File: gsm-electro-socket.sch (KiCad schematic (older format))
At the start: 18 parts, among them IC1 ATMEGA328-P, Q1 BC337, SW1 RESET, U1 PWRCONV, U2 SIM800C, Y1 16Mhz

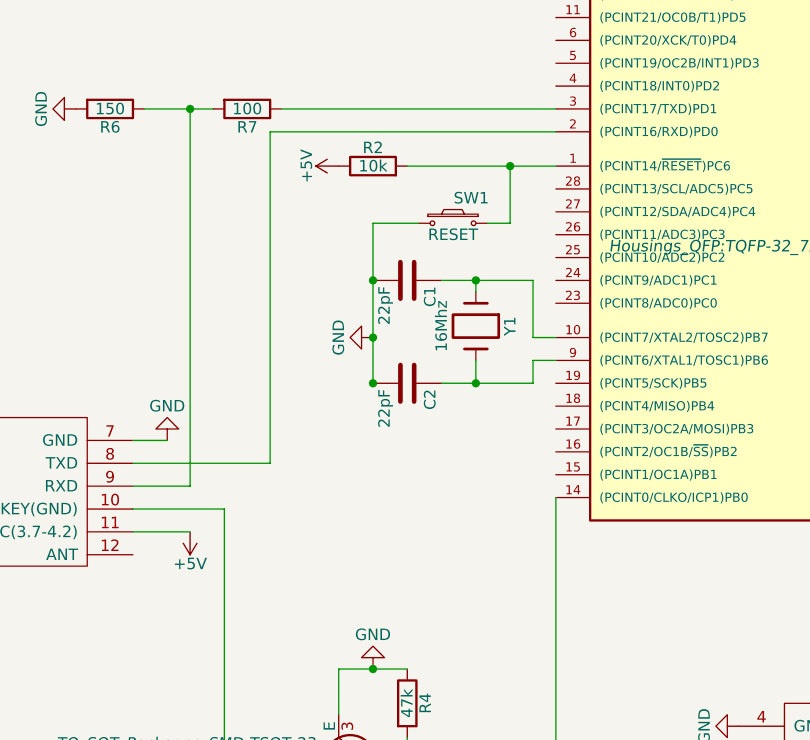
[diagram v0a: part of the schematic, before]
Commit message: update schema
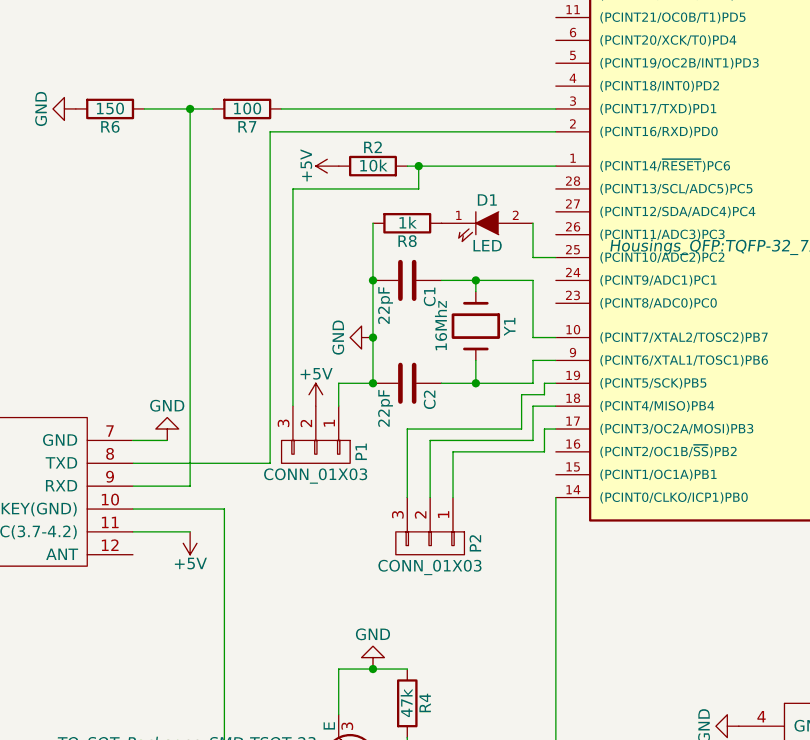
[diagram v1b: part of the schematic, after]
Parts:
- removed SW1: RESET, Buttons_Switches_SMD:SW_DIP_x1_W5.08mm_Slide_Copal_CHS-A, symbol SW_PUSH_SMALL_H
- added D1: LED, LEDs:LED_D2.0mm_W4.0mm_H2.8mm_FlatTop, symbol LED
- added P1, P2: CONN_01X03, Pin_Headers:Pin_Header_Angled_1x03_Pitch2.54mm, symbol CONN_01X03
- added R8: 1k, Resistors_SMD:R_0805_HandSoldering, symbol R
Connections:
- net +5V: now also P1.2 (P2)
- net GND: now also P1.1 (P1), R8.2
- net at IC1.1 ((PCINT14/~RESET~)PC6), R2.2: now also P1.3 (P3)
- net at IC1.17 ((PCINT3/OC2A/MOSI)PB3): now also P2.1 (P1)
- net at IC1.18 ((PCINT4/MISO)PB4): now also P2.2 (P2)
- net at IC1.19 ((PCINT5/SCK)PB5): now also P2.3 (P3)
- net at IC1.25 ((PCINT10/ADC2)PC2): now also D1.2 (A)
- new net: D1.1 (K), R8.1
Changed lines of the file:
@@
-$EndComp
-$Comp
-L SW_PUSH_SMALL_H SW1
-U 1 1 5A398B09
-P 5350 2500
-F 0 "SW1" H 5430 2610 50  0000 C CNN
-F 1 "RESET" H 5350 2450 50  0000 C CNN
-F 2 "Buttons_Switches_SMD:SW_DIP_x1_W5.08mm_Slide_Copal_CHS-A" H 5350 2700 50  0001 C CNN
-F 3 "" H 5350 2700 50  0000 C CNN
-	1    5350 2500
-	1    0    0    -1
 $EndComp
 $Comp
@@
 	5550 4850 5800 4850
 Wire Wire Line
-	5200 2500 5000 2500
-Wire Wire Line
-	5500 2500 5600 2500
-Wire Wire Line
-	5600 2500 5600 2250
-Connection ~ 5600 2250
-Wire Wire Line
 	5700 3200 5700 3100
 Wire Wire Line
@@
 Wire Wire Line
 	7900 3900 8000 3900
-Wire Wire Line
-	5000 2500 5000 3200
 $Comp
 L GND #PWR010
@@
 	0    1    1    0
 $EndComp
+$Comp
+L CONN_01X03 P2
+U 1 1 5A416111
+P 5250 3900
+F 0 "P2" H 5250 4100 50  0000 C CNN
+F 1 "CONN_01X03" V 5350 3900 50  0000 C CNN
+F 2 "Pin_Headers:Pin_Header_Angled_1x03_Pitch2.54mm" H 5250 3900 50  0001 C CNN
+F 3 "" H 5250 3900 50  0000 C CNN
+	1    5250 3900
+	0    1    1    0
+$EndComp
+Wire Wire Line
+	5150 3700 5150 3400
+Wire Wire Line
+	5150 3400 5650 3400
+Wire Wire Line
+	5650 3400 5650 3250
+Wire Wire Line
+	5650 3250 5750 3250
+Wire Wire Line
+	5750 3250 5750 3200
+Wire Wire Line
+	5750 3200 5800 3200
+Wire Wire Line
+	5800 3300 5700 3300
+Wire Wire Line
+	5700 3300 5700 3450
+Wire Wire Line
+	5700 3450 5250 3450
+Wire Wire Line
+	5250 3450 5250 3700
+Wire Wire Line
+	5350 3700 5350 3500
+Wire Wire Line
+	5350 3500 5750 3500
+Wire Wire Line
+	5750 3500 5750 3400
+Wire Wire Line
+	5750 3400 5800 3400
+Wire Wire Line
+	4650 2350 5200 2350
+Wire Wire Line
+	5200 2350 5200 2250
+Connection ~ 5200 2250
+Wire Wire Line
+	5000 3200 4850 3200
+Wire Wire Line
+	4850 3200 4850 3300
+$Comp
+L CONN_01X03 P1
+U 1 1 5A416B6A
+P 4750 3500
+F 0 "P1" H 4750 3700 50  0000 C CNN
+F 1 "CONN_01X03" V 4850 3500 50  0000 C CNN
+F 2 "Pin_Headers:Pin_Header_Angled_1x03_Pitch2.54mm" H 4750 3500 50  0001 C CNN
+F 3 "" H 4750 3500 50  0000 C CNN
+	1    4750 3500
+	0    1    1    0
+$EndComp
+Wire Wire Line
+	5000 2500 5000 3200
+Wire Wire Line
+	4650 3300 4650 2350
+$Comp
+L +5V #PWR014
+U 1 1 5A416D96
+P 4750 3300
+F 0 "#PWR014" H 4750 3150 50  0001 C CNN
+F 1 "+5V" H 4750 3440 50  0000 C CNN
+F 2 "" H 4750 3300 50  0000 C CNN
+F 3 "" H 4750 3300 50  0000 C CNN
+	1    4750 3300
+	1    0    0    -1
+$EndComp
+$Comp
+L R R8
+U 1 1 5A417393
+P 5150 2500
+F 0 "R8" V 5230 2500 50  0000 C CNN
+F 1 "1k" V 5150 2500 50  0000 C CNN
+F 2 "Resistors_SMD:R_0805_HandSoldering" V 5080 2500 50  0001 C CNN
+F 3 "" H 5150 2500 50  0000 C CNN
+	1    5150 2500
+	0    1    1    0
+$EndComp
+$Comp
+L LED D1
+U 1 1 5A4176DA
+P 5500 2500
+F 0 "D1" H 5500 2600 50  0000 C CNN
+F 1 "LED" H 5500 2400 50  0000 C CNN
+F 2 "LEDs:LED_D2.0mm_W4.0mm_H2.8mm_FlatTop" H 5500 2500 50  0001 C CNN
+F 3 "" H 5500 2500 50  0000 C CNN
+	1    5500 2500
+	1    0    0    -1
+$EndComp
+Wire Wire Line
+	5700 2500 5700 2650
+Wire Wire Line
+	5700 2650 5800 2650
 $EndSCHEMATC
